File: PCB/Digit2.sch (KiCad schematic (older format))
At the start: 1 part

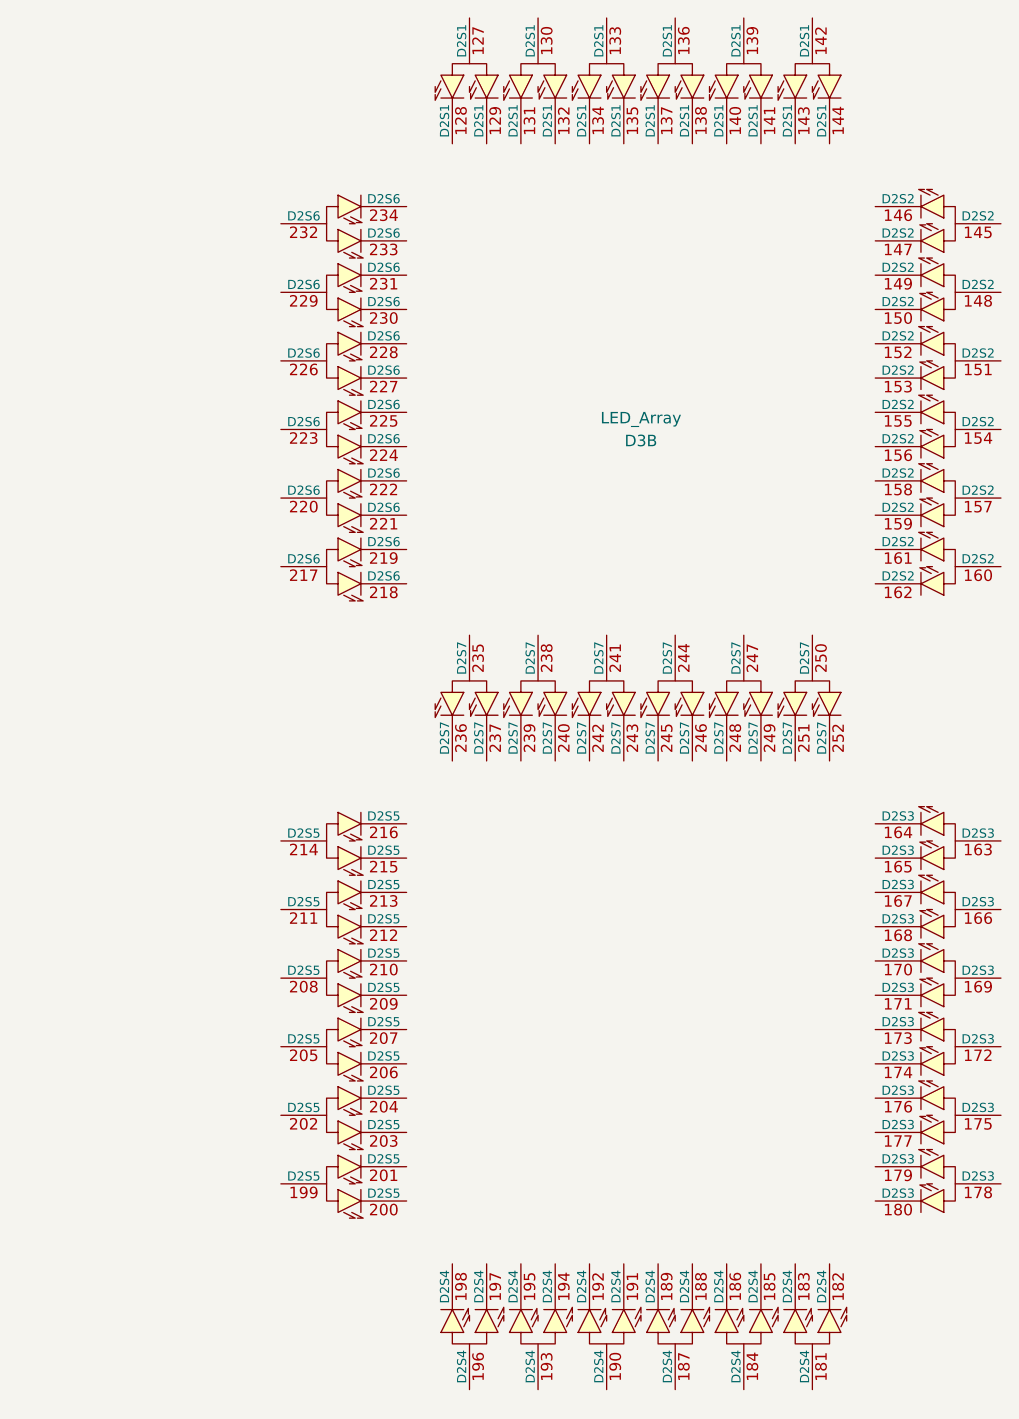
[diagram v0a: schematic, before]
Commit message: Worked on PCB.
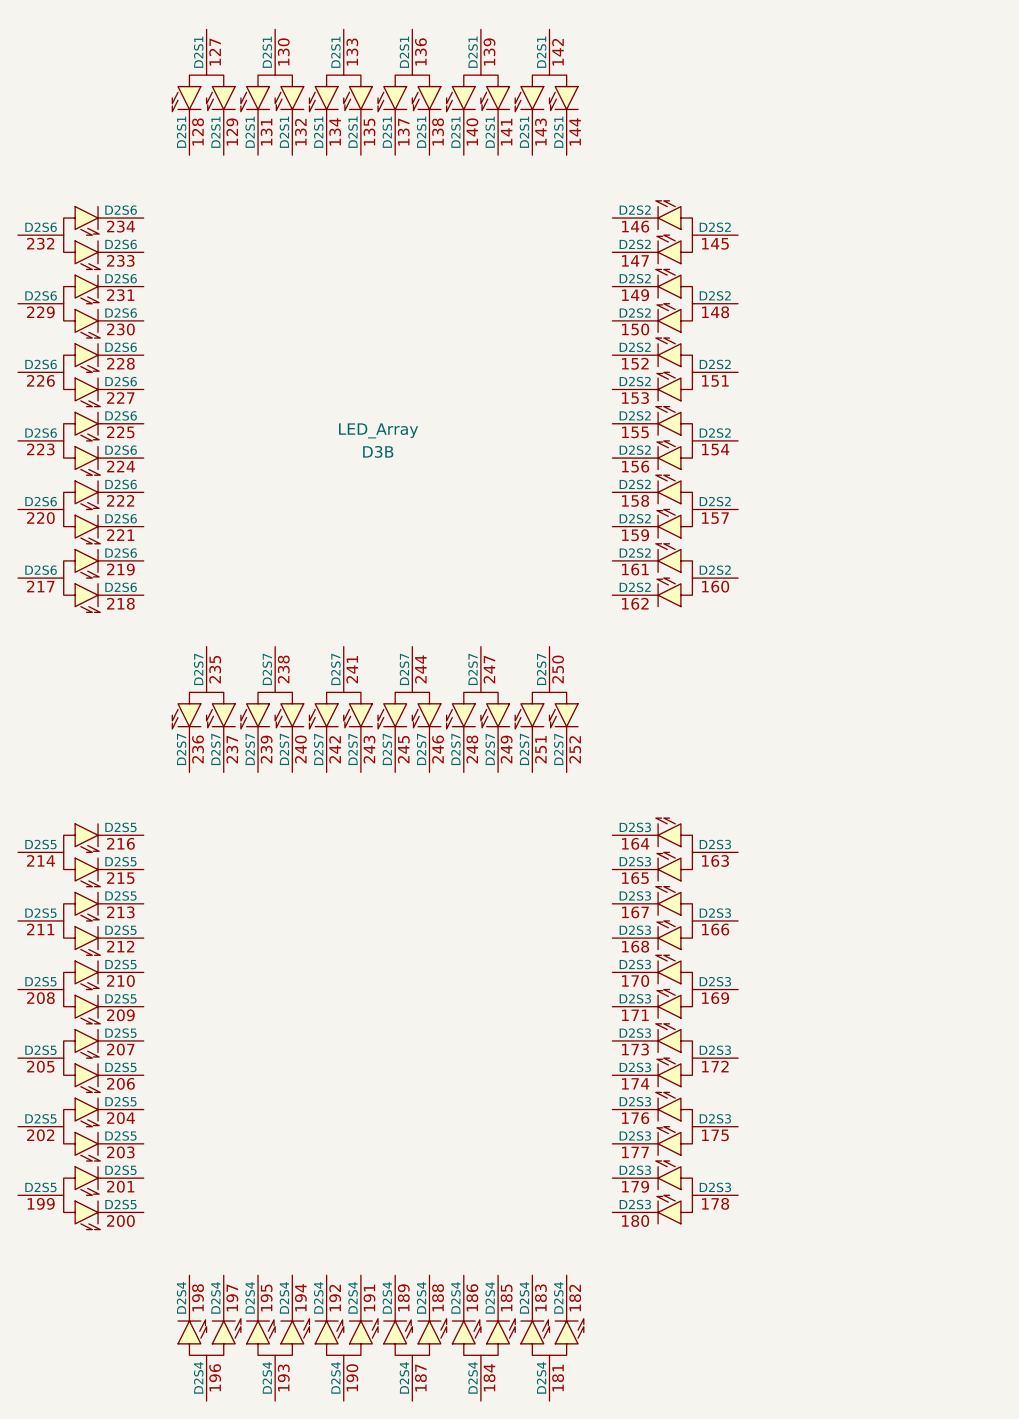
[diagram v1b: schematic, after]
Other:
- moved on the sheet: D3B
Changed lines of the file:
@@
 L LED_Array D3
 U 2 1 54BC7639
-P 4900 4100
-F 0 "D3" H 4900 5250 50  0000 C CNN
-F 1 "LED_Array" H 4900 5350 50  0000 C CNN
-F 2 "Custom:LED-ARRAY" H 4900 5025 50  0001 C CNN
-F 3 "" H 4900 5025 50  0000 C CNN
-	2    4900 4100
+P 3750 4150
+F 0 "D3" H 3750 5300 50  0000 C CNN
+F 1 "LED_Array" H 3750 5400 50  0000 C CNN
+F 2 "Custom:LED-ARRAY" H 3750 5075 50  0001 C CNN
+F 3 "" H 3750 5075 50  0000 C CNN
+	2    3750 4150
 	1    0    0    -1
 $EndComp

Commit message: Updated schematic.
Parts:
- added Q? (x14): FDG1024NZ, SC70-6, symbol FDG1024NZ
- added R? (x14): 10K, symbol R
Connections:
- net labels added: D1A1, D1A2, D1A3, D1A4, D1A5, D1A6, D1S1G, D1S1R, D1S2G, D1S2R, D1S3G, D1S3R, D1S4G, D1S4R, D1S5G, D1S5R, D1S6G, D1S6R, D1S7G, D1S7R, GND
- wire segments 0 -> 257
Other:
- moved on the sheet: D3B
